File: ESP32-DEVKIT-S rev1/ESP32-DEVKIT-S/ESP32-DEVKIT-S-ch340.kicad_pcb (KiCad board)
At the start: 2 copper layers, 28.9 x 42.5 mm, 94 parts, among them J1 JST_2MM_MALE, J2 USB_C_2-LAYER_PADS, J3 Conn_01x20, J4 QWIIC_RIGHT_ANGLE, J5 Conn_01x20, J6 Conn_01x20, J7 QWIIC_RIGHT_ANGLE, Q1 DMG2305UX 20V/4.2A/52mΩ/1.4W, Q2 MBT3904DW1T1, U1 ADXL345, U11 MAX17048, U3 >VALUE, U4 MCP73831, U5 ADS1115IDGS, U6 ADS1115IDGS, U7 ADS1115IDGS, U8 ADS1115IDGS, U9 CH340K

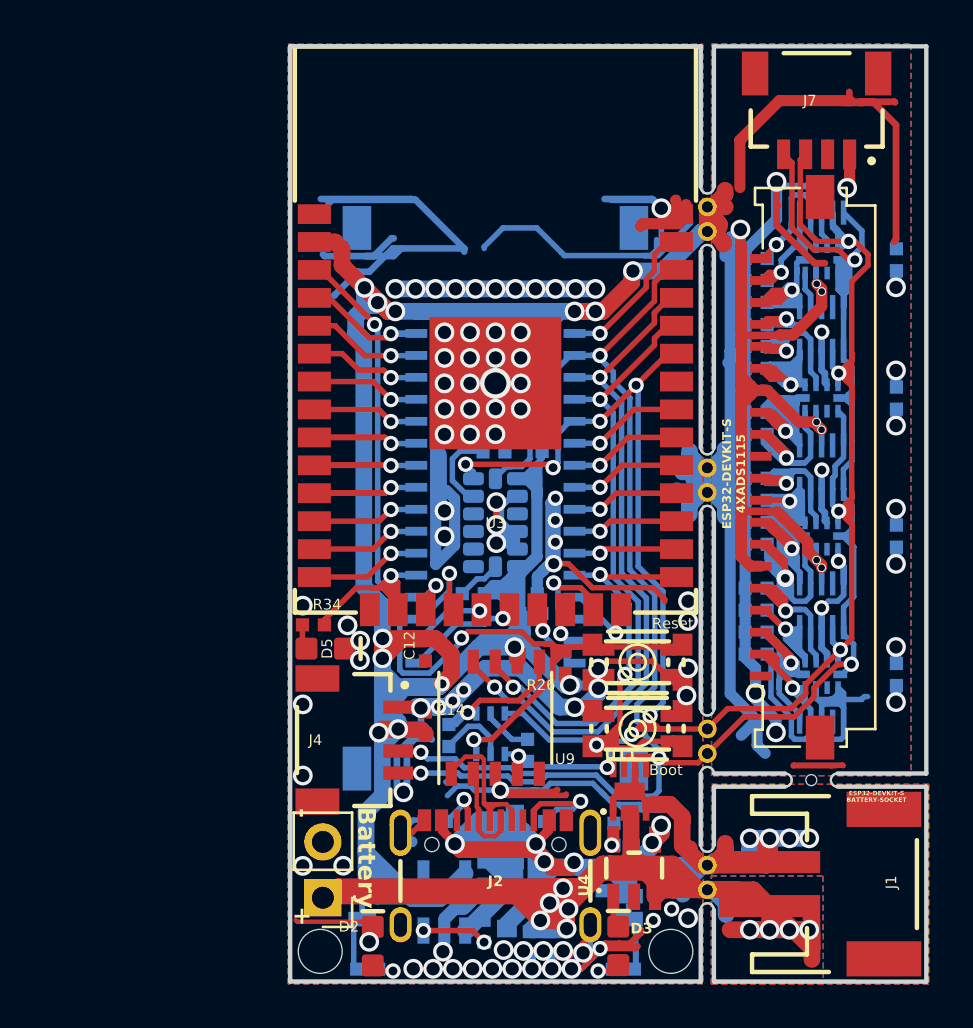
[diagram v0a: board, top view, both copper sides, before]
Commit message: .
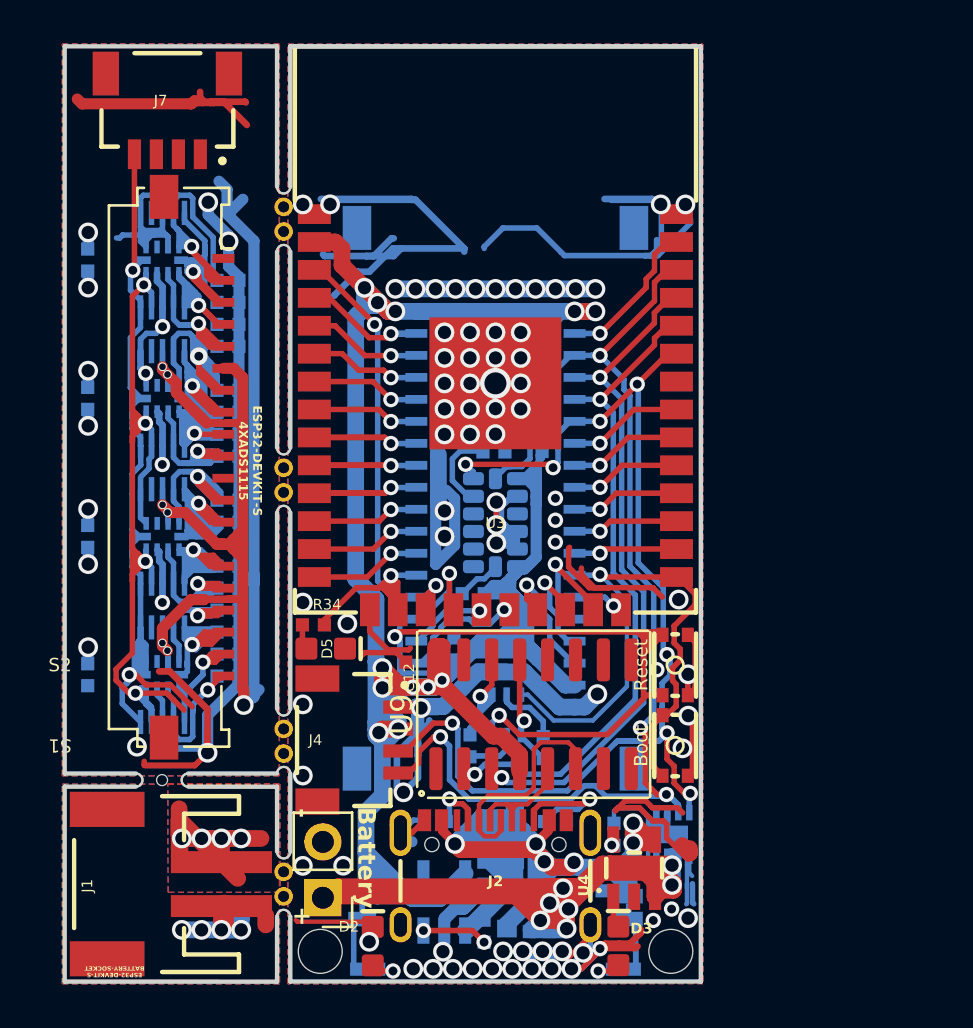
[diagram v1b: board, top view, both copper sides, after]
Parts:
- removed the >NAME at (107.6, 73.8)
- removed the >NAME at (107.6, 70.8)
- removed the >NAME at (116.0, 65.0)
- removed the >NAME at (116.0, 52.5)
- removed the >NAME at (116.0, 71.3)
- removed the >NAME at (116.0, 58.7)
- removed the ? at (115.7, 71.9)
- removed the ? at (115.7, 65.6)
- removed the ? at (115.7, 53.1)
- removed the G*** at (115.4, 81.3)
- removed the G*** at (115.4, 45.8)
- removed the mouse-bite-emm-slot at (110.8, 80.6)
- removed the mouse-bite-emm-slot at (110.8, 62.5)
- removed the mouse-bite-emm-slot at (110.8, 74.4)
- removed the mouse-bite-emm-slot at (110.8, 50.6)
- added >NAME: >VALUE, Silicon-Standard:QFN-10-RSE, B.Cu at (86.0, 71.3)
- added >NAME: >VALUE, Silicon-Standard:QFN-10-RSE, B.Cu at (86.0, 58.8)
- added >NAME: >VALUE, Silicon-Standard:QFN-10-RSE, B.Cu at (86.0, 65.0)
- added >NAME: >VALUE, Silicon-Standard:QFN-10-RSE, B.Cu at (86.0, 52.5)
- added ?: , , F.Cu at (86.2, 51.9)
- added ?: , , F.Cu at (86.2, 70.7)
- added ?: , , F.Cu at (86.3, 58.2)
- added G***: LOGO, logo:Hasatio_logo_mini, B.Cu at (85.9, 45.8)
- added G***: LOGO, logo:Hasatio_logo_mini, B.Cu at (86.9, 80.5)
- added mouse-bite-emm-slot: VAL**, Panelization:mouse-bite-1mm 2, F.Cu at (91.5, 80.9)
- added mouse-bite-emm-slot: VAL**, Panelization:mouse-bite-1mm 2, F.Cu at (91.5, 62.5)
- added mouse-bite-emm-slot: VAL**, Panelization:mouse-bite-1mm 2, F.Cu at (91.5, 50.6)
- added mouse-bite-emm-slot: VAL**, Panelization:mouse-bite-1mm 2, F.Cu at (91.5, 74.4)
- C14, R26, U11: moved to B.Cu
- S1, S2: footprint SparkFun ESP32 Thing Plus C:TACTILE_SWITCH_SMD_4.6X2.8MM -> Switches:TACTILE_SWITCH_SMD_2.8X1.9MM
- U9: value CH340K -> CH340C; footprint Package_SO:SSOP-10_3.9x4.9mm_P1.00mm -> PCM_Package_SO_AKL:SOIC-16_3.9x9.9mm_P1.27mm
- moved C11 41.4 mm to (82.6, 71.3), turned to -90 degrees
- moved C8 41.3 mm to (82.6, 52.5), turned to -90 degrees
- moved C10 37.3 mm to (82.6, 65.0), turned to -90 degrees
- moved C9 37.3 mm to (82.6, 58.8), turned to -90 degrees
- moved U8 35.4 mm to (86.0, 71.3), turned to -90 degrees
- moved U5 35.4 mm to (86.0, 52.5), turned to -90 degrees
- moved J1 32.3 mm to (85.0, 80.9), turned to 90 degrees
- moved U7 30.6 mm to (86.0, 65.0), turned to -90 degrees
- moved U6 30.6 mm to (86.0, 58.8), turned to -90 degrees
- moved R25 30.6 mm to (89.0, 71.4), turned to 180 degrees
- moved J7 29.5 mm to (86.2, 47.7)
- moved mouse-bite-1mm-slot 29.5 mm to (86.0, 76.1)
- moved R10 29.4 mm to (89.0, 53.4), turned to 0 degrees
- moved R24 29.4 mm to (89.0, 70.4), turned to 180 degrees
- moved R11 28.3 mm to (89.0, 54.4), turned to 0 degrees
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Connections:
- S1 pad 2: /GPIO_0/ADC2_1/QPWR -> GND
- S1 pad 3: GND -> /GPIO_0/ADC2_1/QPWR
- S2 pad 2: /~{RESET} -> GND
- S2 pad 3: GND -> /~{RESET}
- U9 pad 1: /D+ -> GND
- U9 pad 10: 3.3V -> unconnected-(U9-~{DSR}-Pad10)
- U9 pad 2: /D- -> /GPIO_3/RX
- U9 pad 3: GND -> /GPIO_1/TX
- U9 pad 4: /CH340-DTR -> 3.3V
- U9 pad 5: unconnected-(U9-~{CTS}-Pad5) -> /D+
- U9 pad 6: /CH340-RTS -> /D-
- U9 pad 7: 3.3V -> unconnected-(U9-NC-Pad7)
- U9 pad 8: /GPIO_3/RX -> unconnected-(U9-NC-Pad8)
- U9 pad 9: /GPIO_1/TX -> unconnected-(U9-~{CTS}-Pad9)
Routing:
- net GND: track 332.3 -> 293.5 mm, vias 96 -> 90
- net /~{RESET}: track 45.3 -> 56.2 mm
- net V_BATT: track 95.1 -> 85.6 mm, vias 9 -> 11
- net /GPIO_21/SDA: track 115.0 -> 107.3 mm
- net /D-: track 5.03 -> 10.7 mm
- net 3.3V: track 241.4 -> 237.2 mm, vias 24 -> 23
- net /GPIO_22/SCL: track 108.1 -> 103.9 mm, vias 5 -> 7
- net /D+: track 9.13 -> 5.94 mm
- net /GPIO_8/SDI: track 1.66 -> 4.71 mm
- net V_USB: track 44.2 -> 47.3 mm
- net /CH340-DTR: track 2.15 -> 4.92 mm
- net /GPIO_7/SDO: track 3.21 -> 5.81 mm
- net /GPIO_3/RX: track 28.1 -> 30.2 mm
- net /GPIO_0/ADC2_1/QPWR: track 26.2 -> 28.2 mm, vias 3 -> 1
- net Net-(J2-CC2): track 4.77 -> 6.22 mm
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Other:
- board size 28.9 x 42.5 mm -> 28.9 x 42.6 mm
- board text added: "S1"
- board text added: "S2"

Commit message: .
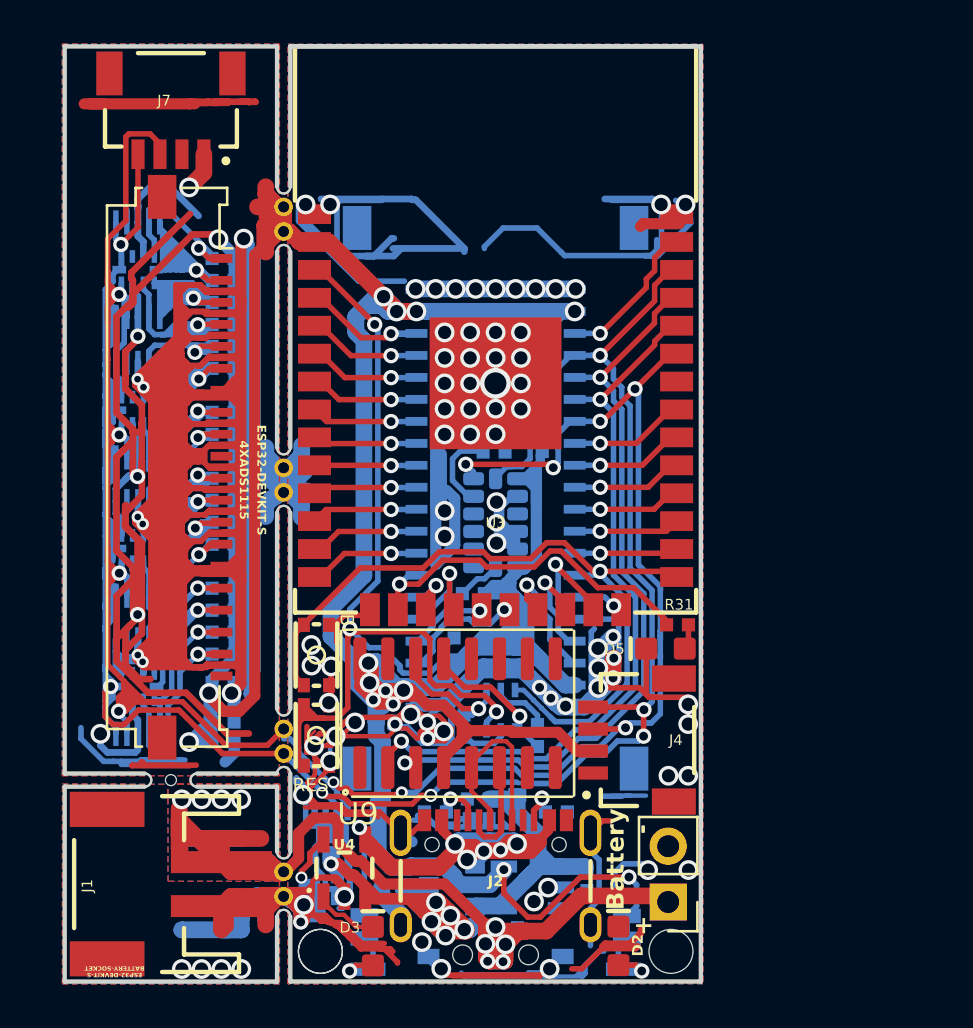
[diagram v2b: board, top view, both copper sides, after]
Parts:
- removed the >NAME at (86.0, 71.3)
- removed the >NAME at (86.0, 58.8)
- removed the >NAME at (86.0, 65.0)
- removed the >NAME at (86.0, 52.5)
- removed the ? at (86.2, 51.9)
- removed the ? at (93.2, 83.9)
- removed the ? at (109.1, 83.9)
- removed the ? at (86.2, 70.7)
- removed the ? at (86.3, 58.2)
- removed the G*** at (105.3, 46.2)
- removed the G*** at (85.9, 45.8)
- removed the G*** at (86.9, 80.5)
- removed R32, R33: 5.1k, SparkFun ESP32 Thing Plus C:0402-TIGHT
- removed R34: 1k, SparkFun ESP32 Thing Plus C:0402-TIGHT
- added >NAME: >VALUE, Silicon-Standard:QFN-10-RSE, B.Cu at (84.9, 59.3)
- added >NAME: >VALUE, Silicon-Standard:QFN-10-RSE, B.Cu at (84.9, 52.9)
- added >NAME: >VALUE, Silicon-Standard:QFN-10-RSE, B.Cu at (84.9, 65.6)
- added >NAME: >VALUE, Silicon-Standard:QFN-10-RSE, B.Cu at (84.9, 71.9)
- added ? (x2): , , F.Cu at (93.2, 83.9)
- added ?: , , F.Cu at (109.1, 83.9)
- added G***: LOGO, logo:Hasatio_logo_mini, B.Cu at (86.3, 80.9)
- added G***: LOGO, logo:Hasatio_logo_mini, B.Cu at (96.4, 46.2)
- added G***: LOGO, logo:Hasatio_logo_mini, B.Cu at (86.3, 45.8)
- added R29: 5.1k, SparkFun ESP32 Thing Plus C:0402-TIGHT, B.Cu at (103.9, 77.6)
- added R30: 5.1k, SparkFun ESP32 Thing Plus C:0402-TIGHT, B.Cu at (98.4, 77.6)
- added R31: 1k, SparkFun ESP32 Thing Plus C:0402-TIGHT, F.Cu at (109.4, 69.1)
- added SW1: ON OFF, Button_Switch_SMD:SW_SPDT_k3-1295, B.Cu at (101.2, 84.1)
- C12: moved to B.Cu
- S1: value Boot -> B
- S2: value Reset -> RES
- moved C8 22.8 mm to (88.8, 74.4), turned to 0 degrees
- moved U5 19.4 mm to (84.9, 71.9)
- moved R25 19.0 mm to (88.8, 52.4)
- moved U8 18.5 mm to (84.9, 52.9)
- moved R10 17.0 mm to (88.8, 70.4)
- moved R24 17.0 mm to (88.8, 53.4)
- moved S1 16.8 mm to (93.0, 70.4)
- moved S2 16.6 mm to (93.0, 74.1)
- moved C9 16.0 mm to (88.8, 73.5), turned to 0 degrees
- moved REF** 15.7 mm to (109.0, 81.7)
- moved U11 15.5 mm to (93.7, 78.6)
- moved D5 15.5 mm to (108.9, 70.1), turned to 180 degrees
- moved R11 15.0 mm to (88.8, 69.4)
- moved R23 15.0 mm to (88.8, 54.4)
- moved R28 14.3 mm to (92.5, 81.4), turned to 90 degrees
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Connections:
- J1 pad 2: V_BATT -> /V
- J6 pad 1: unconnected-(J6-Pin_1-Pad1) -> /A16
- J6 pad 10: /A8 -> unconnected-(J6-Pin_10-Pad10)
- J6 pad 11: unconnected-(J6-Pin_11-Pad11) -> /A8
- J6 pad 12: /A9 -> /A7
- J6 pad 13: /A10 -> /A6
- J6 pad 14: GND -> /A5
- J6 pad 15: /A11 -> GND
- J6 pad 16: /A12 -> /A4
- J6 pad 17: /A13 -> /A3
- J6 pad 18: /A14 -> /A2
- J6 pad 19: /A15 -> /A1
- J6 pad 2: /A1 -> /A15
- J6 pad 20: /A16 -> unconnected-(J6-Pin_20-Pad20)
- J6 pad 3: /A2 -> /A14
- J6 pad 4: /A3 -> /A13
- J6 pad 5: /A4 -> /A12
- J6 pad 6: GND -> /A11
- J6 pad 7: /A5 -> GND
- J6 pad 8: /A6 -> /A10
- J6 pad 9: /A7 -> /A9
- REF** pad 1: V_BATT -> /V
- U2 pad 4: unconnected-(U2-NC-Pad4) -> VIN
- U5 pad 4: /A1 -> /A4
- U5 pad 5: /A2 -> /A3
- U5 pad 6: /A3 -> /A2
- U5 pad 7: /A4 -> /A1
- U6 pad 4: /A5 -> /A8
- U6 pad 5: /A6 -> /A7
- U6 pad 6: /A7 -> /A6
- U6 pad 7: /A8 -> /A5
- U7 pad 4: /A9 -> /A12
- U7 pad 5: /A10 -> /A11
- U7 pad 6: /A11 -> /A10
- U7 pad 7: /A12 -> /A9
- U8 pad 4: /A13 -> /A16
- U8 pad 5: /A14 -> /A15
- U8 pad 6: /A15 -> /A14
- U8 pad 7: /A16 -> /A13
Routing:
- net GND: track 293.5 -> 672.7 mm, vias 90 -> 87
- net 3.3V: track 237.2 -> 342.0 mm, vias 23 -> 19
- net /V: track 0.00 -> 64.2 mm, vias 0 -> 9
- net V_BATT: track 85.6 -> 36.5 mm, vias 11 -> 6
- net /GPIO_22/SCL: track 103.9 -> 140.1 mm
- net /GPIO_21/SDA: track 107.3 -> 130.5 mm, vias 12 -> 11
- net /A5: track 24.7 -> 8.36 mm
- net /A6: track 29.2 -> 14.1 mm
- net V_USB: track 47.3 -> 33.6 mm
- net /A2: track 20.7 -> 8.19 mm
- net /A7: track 22.3 -> 32.9 mm
- net /GPIO_0/ADC2_1/QPWR: track 28.2 -> 36.6 mm
- net /A9: track 16.9 -> 8.61 mm
- net /~{RESET}: track 56.2 -> 48.0 mm
- net /A15: track 10.5 -> 18.7 mm
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- added copper zone on B.Cu, net /V
- added copper zone on F.Cu, net /V
- removed copper zone on B.Cu, net V_BATT
- removed copper zone on F.Cu, net V_BATT
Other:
- board size 28.9 x 42.6 mm -> 28.9 x 42.5 mm
- board text added: "C1"
- board text removed: "S1"
- board text removed: "S2"
